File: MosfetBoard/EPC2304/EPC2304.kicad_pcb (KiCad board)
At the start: 2 copper layers, 120 x 75 mm, 179 parts, among them J10 DriverConn, J14 BATT-Conn2, J4 PhaseConn, J5 PhaseConn, J6 PhaseConn, J7 DriverConn, J8 DriverConn, J9 BATT-Conn1, Q1 EPC2304, Q13 EPC2304, Q14 EPC2304, Q15 EPC2304, Q2 EPC2304, Q3 EPC2304, Q4 EPC2304, Q5 EPC2304, Q6 EPC2304, Q7 EPC2304, Q8 EPC2304, Q9 EPC2304, U1 2EDF7275KXUMA1, U2 2EDF7275KXUMA1, U3 2EDF7275KXUMA1

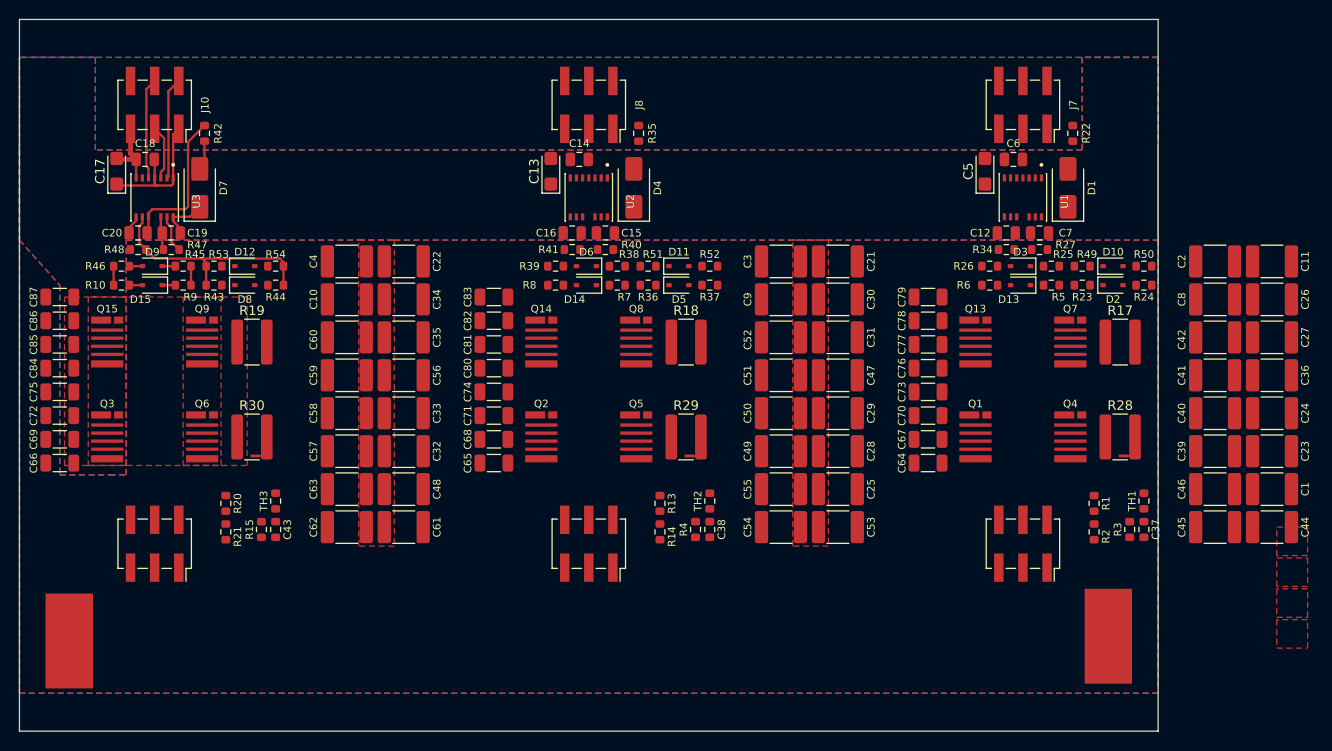
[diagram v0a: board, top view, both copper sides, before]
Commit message: v2.6.2 - EPC2304
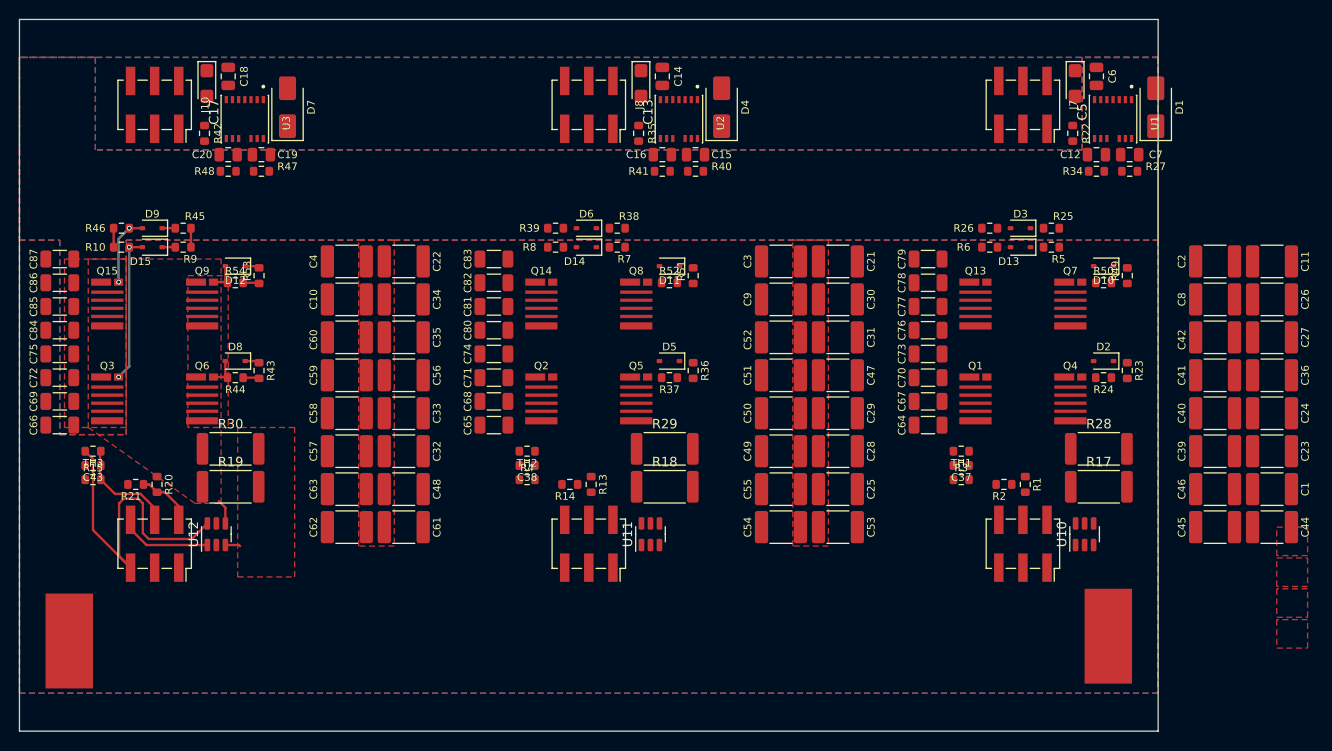
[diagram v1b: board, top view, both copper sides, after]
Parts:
- removed JP1, JP2, JP3: DummyJumper, GigaVescLibs:SolderJumper0.3mm
- added U10: INA181, Package_TO_SOT_SMD:SOT-23-6, F.Cu at (208.2, 108.2)
- added U11: INA181, Package_TO_SOT_SMD:SOT-23-6, F.Cu at (162.5, 108.2)
- added U12: INA181, Package_TO_SOT_SMD:SOT-23-6, F.Cu at (116.8, 108.2)
- R17, R18, R19, R28, R29, R30: footprint Resistor_SMD:R_1218_3246Metric_Pad1.22x4.75mm_HandSolder -> Resistor_SMD:R_2512_6332Metric
- moved C37 20.4 mm to (195.2, 101.0), turned to 180 degrees
- moved C38 20.4 mm to (149.5, 101.0), turned to 180 degrees
- moved C43 20.4 mm to (103.8, 101.0), turned to 180 degrees
- moved TH1 20.0 mm to (195.2, 99.5), turned to 0 degrees
- moved TH2 20.0 mm to (149.5, 99.5), turned to 0 degrees
- moved TH3 20.0 mm to (103.8, 99.5), turned to 0 degrees
- moved R15 18.5 mm to (103.8, 102.5), turned to 180 degrees
- moved R3 18.5 mm to (195.2, 102.5), turned to 180 degrees
- moved R4 18.5 mm to (149.5, 102.5), turned to 180 degrees
- moved R17 15.4 mm to (209.8, 103.2)
- moved R18 15.4 mm to (164.0, 103.2)
- moved R19 15.4 mm to (118.2, 103.2)
- moved C13 13.3 mm to (161.5, 60.8), turned to -90 degrees
- moved C17 13.3 mm to (115.8, 60.8), turned to -90 degrees
- moved C5 13.3 mm to (207.2, 60.8), turned to -90 degrees
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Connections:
- C14 pad 1: /PhaseMosfets2/3.3V_IN -> -BATT
- C14 pad 2: -BATT -> /PhaseMosfets2/3.3V_IN
- C18 pad 1: /PhaseMosfets3/3.3V_IN -> -BATT
- C18 pad 2: -BATT -> /PhaseMosfets3/3.3V_IN
- C6 pad 1: /PhaseMosfets1/3.3V_IN -> -BATT
- C6 pad 2: -BATT -> /PhaseMosfets1/3.3V_IN
- J4 pad 3: /PhaseMosfets1/SH- -> -BATT
- J5 pad 3: /PhaseMosfets2/SH- -> -BATT
- J6 pad 3: /PhaseMosfets3/SH- -> -BATT
- Q4 pad 2: /PhaseMosfets1/SH+ -> -BATT
- Q4 pad 4: /PhaseMosfets1/SH+ -> -BATT
- Q4 pad 6: /PhaseMosfets1/SH+ -> -BATT
- Q5 pad 2: /PhaseMosfets2/SH+ -> -BATT
- Q5 pad 4: /PhaseMosfets2/SH+ -> -BATT
- Q5 pad 6: /PhaseMosfets2/SH+ -> -BATT
- Q6 pad 2: /PhaseMosfets3/SH+ -> -BATT
- Q6 pad 4: /PhaseMosfets3/SH+ -> -BATT
- Q6 pad 6: /PhaseMosfets3/SH+ -> -BATT
- Q7 pad 2: /PhaseMosfets1/SH+ -> -BATT
- Q7 pad 4: /PhaseMosfets1/SH+ -> -BATT
- Q7 pad 6: /PhaseMosfets1/SH+ -> -BATT
- Q8 pad 2: /PhaseMosfets2/SH+ -> -BATT
- Q8 pad 4: /PhaseMosfets2/SH+ -> -BATT
- Q8 pad 6: /PhaseMosfets2/SH+ -> -BATT
- Q9 pad 2: /PhaseMosfets3/SH+ -> -BATT
- Q9 pad 4: /PhaseMosfets3/SH+ -> -BATT
- Q9 pad 6: /PhaseMosfets3/SH+ -> -BATT
- R17 pad 1: /PhaseMosfets1/SH+ -> /PhaseMosfets1/PHASE
- R17 pad 2: -BATT -> Net-(U10-+)
- R18 pad 1: /PhaseMosfets2/SH+ -> /PhaseMosfets2/PHASE
- R18 pad 2: -BATT -> Net-(U11-+)
- R19 pad 1: /PhaseMosfets3/SH+ -> /PhaseMosfets3/PHASE
- R19 pad 2: -BATT -> Net-(U12-+)
- R28 pad 1: /PhaseMosfets1/SH+ -> /PhaseMosfets1/PHASE
- R28 pad 2: -BATT -> Net-(U10-+)
- R29 pad 1: /PhaseMosfets2/SH+ -> /PhaseMosfets2/PHASE
- R29 pad 2: -BATT -> Net-(U11-+)
- R30 pad 1: /PhaseMosfets3/SH+ -> /PhaseMosfets3/PHASE
- R30 pad 2: -BATT -> Net-(U12-+)
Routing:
- net /PhaseMosfets3/3.3V_IN2: track 0.00 -> 35.3 mm
- net /PhaseMosfets3/PL: track 24.3 -> 3.41 mm
- net /PhaseMosfets3/12V_IN: track 15.9 -> 0.00 mm
- net -BATT: track 15.1 -> 0.00 mm
- net Net-(D15-A): track 1.38 -> 15.5 mm, vias 0 -> 2
- net /PhaseMosfets3/MOS_TEMP: track 0.00 -> 11.2 mm
- net /PhaseMosfets3/H: track 10.7 -> 0.00 mm
- net /PhaseMosfets3/DISABLE: track 10.7 -> 0.00 mm
- net /PhaseMosfets3/SH+: track 0.00 -> 9.76 mm
- net /PhaseMosfets3/3.3V_IN: track 7.52 -> 0.00 mm
- net Net-(D9-A): track 1.38 -> 7.52 mm, vias 0 -> 2
- net /PhaseMosfets3/V_SENSE: track 0.00 -> 6.10 mm
- net /PhaseMosfets3/L: track 5.74 -> 0.00 mm
- net Net-(D7-K): track 5.25 -> 0.00 mm
- net /PhaseMosfets3/PH: track 7.98 -> 4.00 mm
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- added copper zone on F.Cu, net Net-(U12-+)
- removed copper zone on F.Cu, net /PhaseMosfets3/SH+
